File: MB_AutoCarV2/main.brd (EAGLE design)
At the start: 228.6 x 141.9 mm, 44 parts, among them K1 CQ1-12V, K2 CQ1-12V, K3 CQ1-12V, K4 CQ1-12V, Q1 PN2222, Q2 PN2222, Q3 PN2222, Q4 PN2222, U1 ARDUINO-MEGAFULL

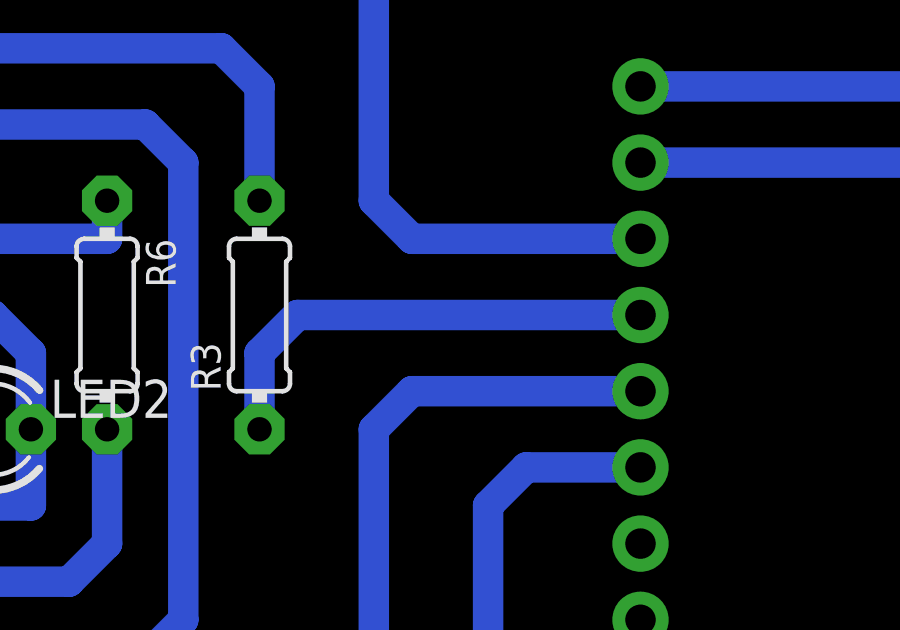
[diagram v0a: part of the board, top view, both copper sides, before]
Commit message: update
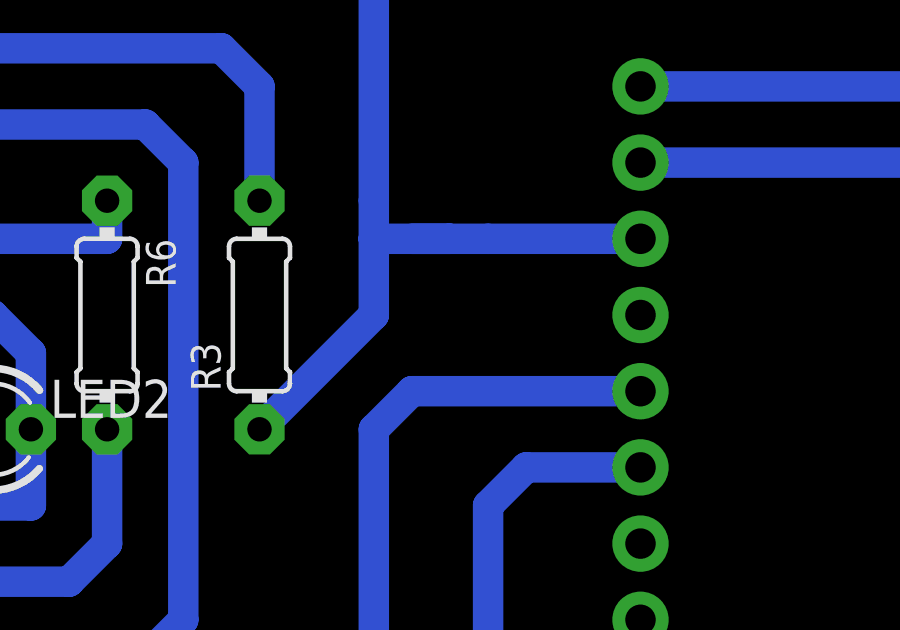
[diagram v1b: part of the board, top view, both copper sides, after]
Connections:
- removed net IN2: R3.1, U1.4
- net IN1: now also R3.1
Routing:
- net IN2: track 15.8 -> 0.00 mm
- net IN1: track 27.7 -> 37.7 mm
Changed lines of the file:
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@@
 <setting verticaltext="up"/>
 </settings>
-<grid distance="50" unitdist="mil" unit="mil" style="lines" multiple="1" display="yes" altdistance="5" altunitdist="mil" altunit="mil"/>
+<grid distance="50" unitdist="mil" unit="mm" style="lines" multiple="1" display="no" altdistance="5" altunitdist="mil" altunit="mil"/>
 <layers>
 <layer number="1" name="Top" color="4" fill="1" visible="no" active="yes"/>
@@
 <wire x1="71.12" y1="85.09" x2="72.39" y2="83.82" width="1.016" layer="16"/>
 <wire x1="72.39" y1="83.82" x2="72.39" y2="69.85" width="1.016" layer="16"/>
-<wire x1="72.39" y1="69.85" x2="73.66" y2="68.58" width="1.016" layer="16"/>
-<wire x1="73.66" y1="68.58" x2="81.28" y2="68.58" width="1.016" layer="16"/>
-</signal>
-<signal name="IN2">
+<wire x1="73.66" y1="68.58" x2="74.93" y2="68.58" width="1.016" layer="16"/>
 <contactref element="R3" pad="1"/>
-<contactref element="U1" pad="4"/>
-<wire x1="81.28" y1="66.04" x2="69.85" y2="66.04" width="1.016" layer="16"/>
-<wire x1="69.85" y1="66.04" x2="68.58" y2="64.77" width="1.016" layer="16"/>
-<wire x1="68.58" y1="64.77" x2="68.58" y2="62.23" width="1.016" layer="16"/>
+<wire x1="74.93" y1="68.58" x2="76.2" y2="68.58" width="1.016" layer="16"/>
+<wire x1="76.2" y1="68.58" x2="81.28" y2="68.58" width="1.016" layer="16"/>
+<wire x1="68.58" y1="62.23" x2="72.39" y2="66.04" width="1.016" layer="16"/>
+<wire x1="72.39" y1="66.04" x2="72.39" y2="68.58" width="1.016" layer="16"/>
+<wire x1="72.39" y1="68.58" x2="72.39" y2="69.85" width="1.016" layer="16"/>
+<wire x1="72.39" y1="68.58" x2="74.93" y2="68.58" width="1.016" layer="16"/>
 </signal>
 <signal name="N$4">
